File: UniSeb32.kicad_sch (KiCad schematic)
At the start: 68 parts, among them IC1 WEMOS-D1-MINI, IC2 GY-BME280-3.3, IC3 AMS1117-3.3, IC4 MCP23008SS, IC5 RT9400, IC6 AMS5915, J1 22-?-0327-2031, J2 ARJM11C7-114-BA-EW2, U1 ESP32-WROOM-32, U2 LAN8720A, X1 AK500{slash}2, X2 AK500{slash}2, X3 233-503, X5 233-504, X61 JST-XH-05-PIN-LONG-PAD, X8 233-508

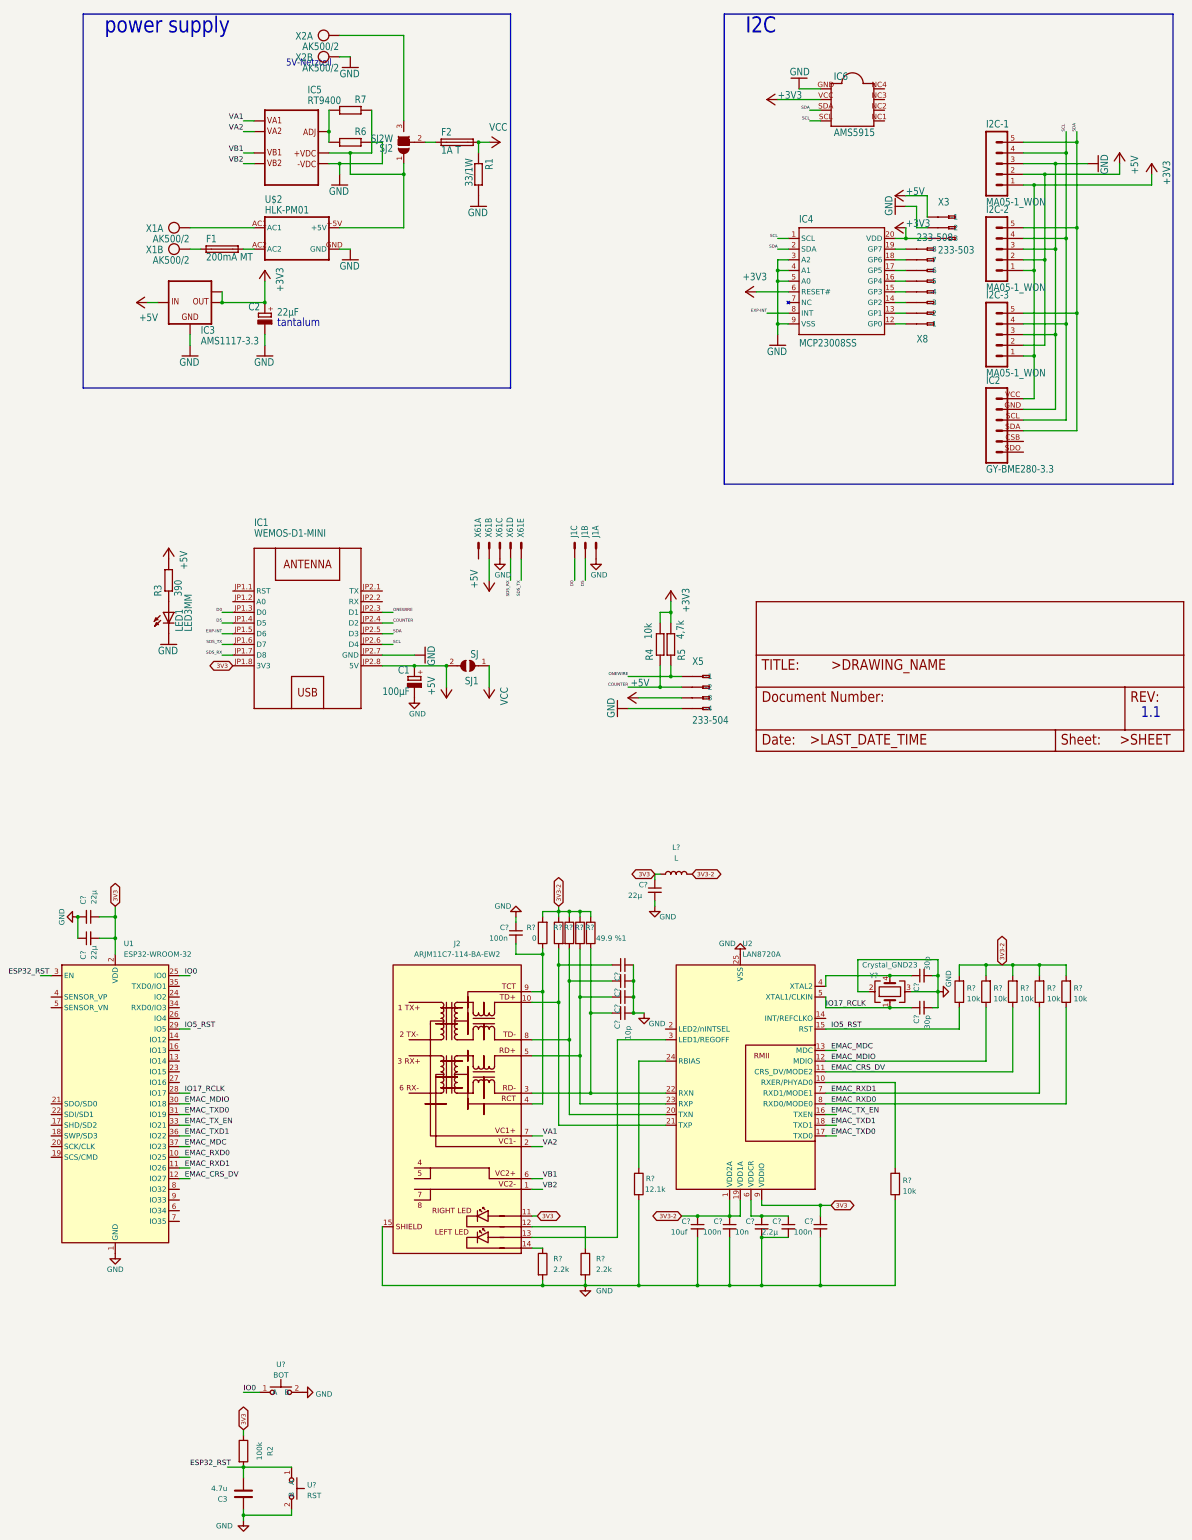
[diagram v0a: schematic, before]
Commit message: .
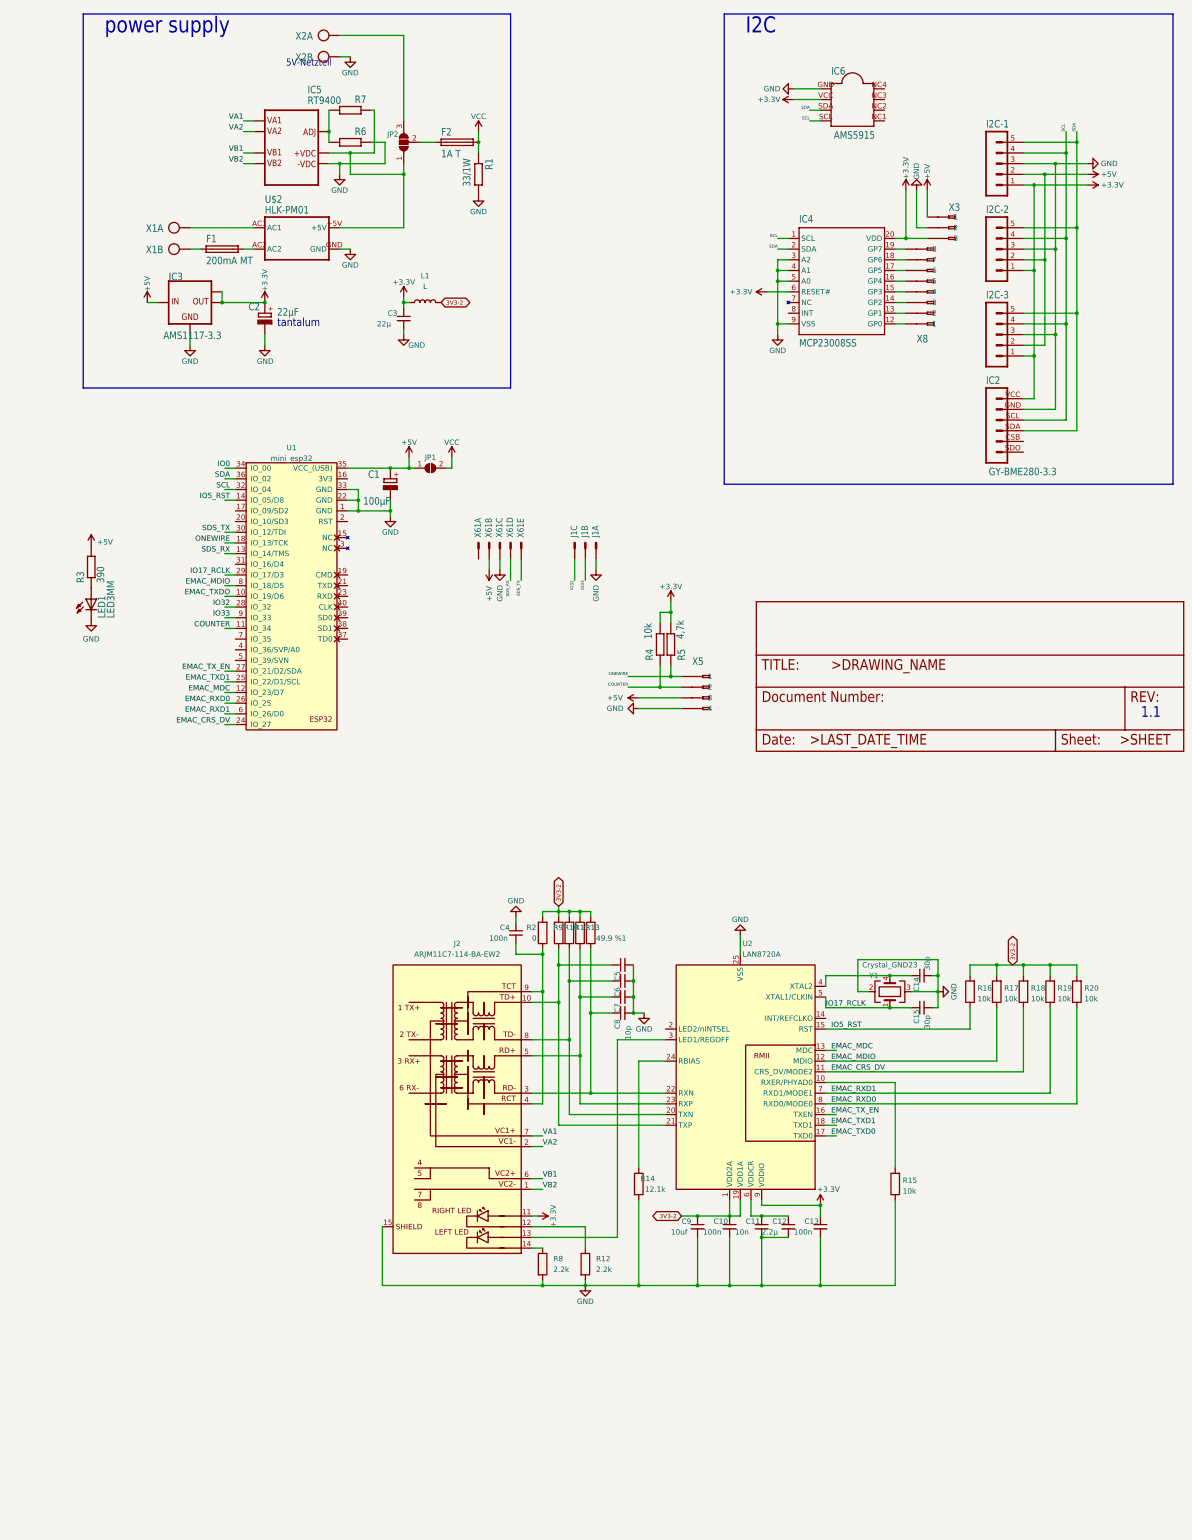
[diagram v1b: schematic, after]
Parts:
- removed C3: 4.7u, symbol Device:C
- removed C? (x2): 22µ, symbol Device:C_Small
- removed IC1: WEMOS-D1-MINI, UniSeb8266:WEMOS-D1-MINI, symbol UniSeb8266-eagle-import:WEMOS-D1-MINI
- removed R2: 100k, Resistor_SMD:R_0603_1608Metric, symbol Device:R
- removed SJ1: SJ, UniSeb8266:SJ, symbol UniSeb8266-eagle-import:SJ
- removed SJ2: SJ2W, UniSeb8266:SJ_2, symbol UniSeb8266-eagle-import:SJ2W
- removed U1: ESP32-WROOM-32, RF_Module:ESP32-WROOM-32, symbol RF_Module:ESP32-WROOM-32
- removed U?: BOT, Switches-Custom:Tactile Push Button 3X6X2.5mm, symbol Switches-Custom:SMD-Switch
- removed U?: RST, Switches-Custom:Tactile Push Button 3X6X2.5mm, symbol Switches-Custom:SMD-Switch
- added JP1: SolderJumper_2_Open, symbol Jumper:SolderJumper_2_Open
- added JP2: SolderJumper_3_Open, Jumper:SolderJumper-3_P1.3mm_Open_Pad1.0x1.5mm_NumberLabels, symbol Jumper:SolderJumper_3_Open
- added U1: mini_esp32, ESP32_mini:ESP32_mini, symbol ESP32_mini:mini_esp32
- gave numbers to parts that had none: 29
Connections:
- net 3V3 is gone; now on net +3.3V: C13.1, C3.1, J2.11 (RLED+), L1.1, U2.9 (VDDIO)
- net +5V: now also JP1.1 (A), U1.35 (VCC_(USB))
- net COUNTER: now also U1.11 (IO_34)
- net EMAC_CRS_DV: now also U1.24 (IO_27)
- net EMAC_MDC: now also U1.12 (IO_23/D7)
- net EMAC_MDIO: now also U1.8 (IO_18/D5)
- net EMAC_RXD0: now also U1.26 (IO_25)
- net EMAC_RXD1: now also U1.6 (IO_26/D0)
- net EMAC_TXD1: now also U1.25 (IO_22/D1/SCL)
- net EMAC_TX_EN: now also U1.27 (IO_21/D2/SDA)
- net GND: now also U1.1 (GND), U1.22 (GND), U1.33 (GND)
- net IO0: now also U1.34 (IO_00)
- net IO17_RCLK: now also U1.29 (IO_17/D3)
- net IO5_RST: now also U1.14 (IO_05/D8)
- net ONEWIRE: now also U1.18 (IO_13/TCK)
- net SCL: now also U1.32 (IO_04)
- net SDA: now also U1.36 (IO_02)
- net SDS_RX: now also U1.13 (IO_14/TMS)
- net SDS_TX: now also U1.30 (IO_12/TDI)
- net VCC: now also JP1.2 (B)
- net at IC5.P$6 (+VDC), R7.1, U$2.+5V: now also JP2.1 (A)
- net at F2.1: now also JP2.2 (C)
- net at X2.1 (KL): now also JP2.3 (B)
- net +3V3 renamed +3.3V
- net D0 renamed IO32
- net IO32: now also U1.28 (IO_32)
- net D5 renamed IO33
- net IO33: now also U1.9 (IO_33)
- net EXP-INT: no longer names the net of IC4.8 (INT)
- new net EMAC_TXDO: U1.10 (IO_19/D6)
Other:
- moved on the sheet: C1, C3, L1, LED1, R16, R17, R18, R19, R20, R3
